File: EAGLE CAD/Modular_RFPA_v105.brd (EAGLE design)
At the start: 152.4 x 152.4 mm, 197 parts, among them IC201 74AHC1G14DBV, IC202 LM324D, J1 FUSE_2P, J2 KK_PCFAN, Q1 IRF630, Q101 IRF630, Q102 IRF520N, Q2 IRF630, Q201 BSS123, T1 HP4_TRAFO, T2 HP4_TRAFO, X101 HEATSINK_OMNI_DUAL30-75-D

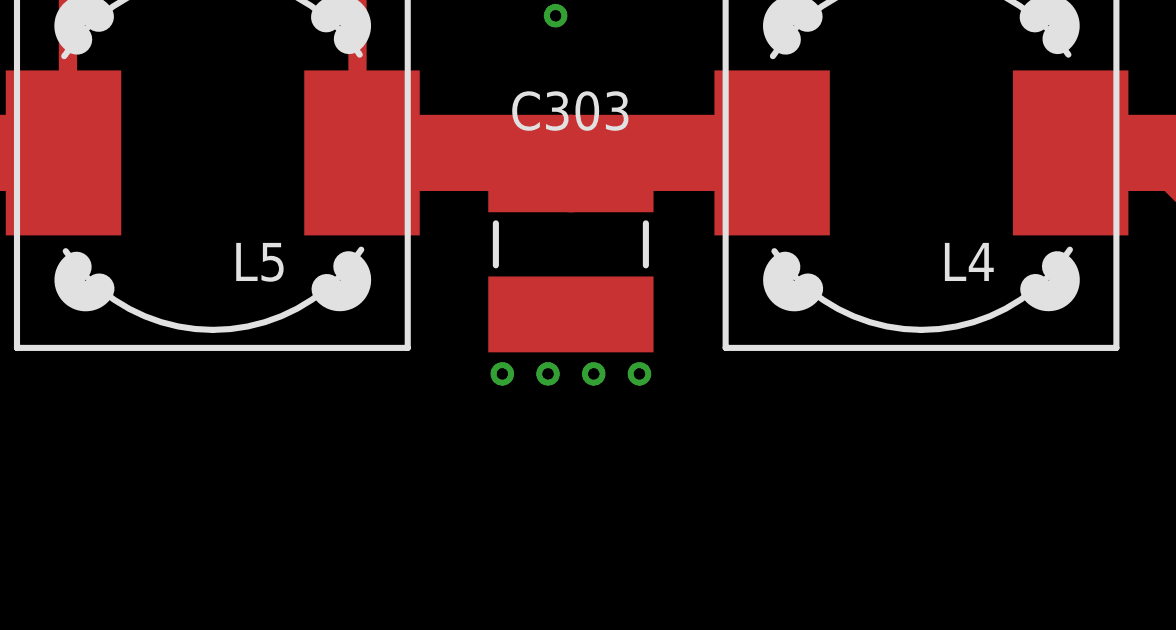
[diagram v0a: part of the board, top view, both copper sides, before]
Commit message: Work on libraries...
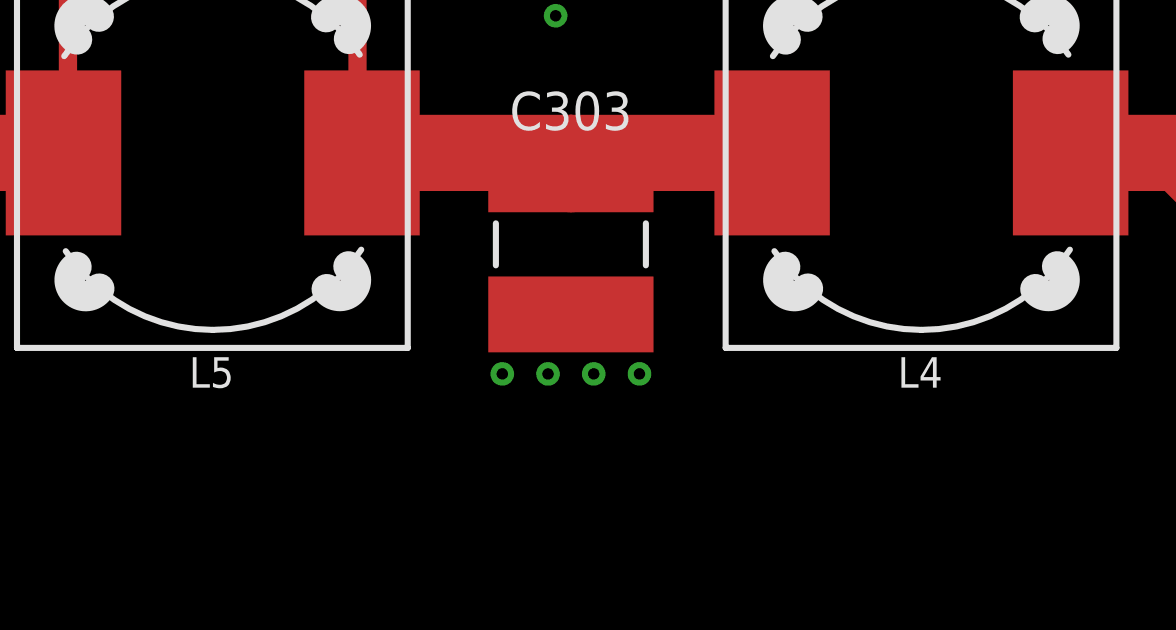
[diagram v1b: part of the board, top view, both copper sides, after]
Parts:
- C1, C111, C112, C7: value 2.2nF -> 22nF
- C102, C104, C12, C6: value 22nF -> 0.1uF
- C103, C11, C5: value 27nF -> 0.1uF
- C105: value 12nF -> 0.1uF
- C106, C107, C109, C110, C17, C207, C208, C24, C26, C27, C28: value DNP -> 0.1uF
- C113, C114, C2, C8: value 10nF -> 0.1uF
- C15, C16: value 4.7uF -> 47nF
- C209: value 15pF -> 0.1uF
- C25: value 1.5nF -> 0.1uF
- C29: value 100nF -> 0.1uF
- L1, L101, L2: value 47nH -> 1uH
- L102: value 150nH -> 1uH
- L4, L5: device inductors:DR127 -> MDT_L:DR127
- R1, R118, R120, R14: value 270 -> 1K
- R101, R105, R13, R18, R26, R5: value 75 -> 1K
- R102, R106: value 150 -> 1K
- R103, R19, R6: value 4.99 -> 1K
- R104: value 10 -> 1K
- R107, R109, R12, R218, R25: value 100 -> 1.0K
- R108, R110, R17, R4: value 100 -> 1K
- R111, R112, R115, R116, R211, R214: value DNP -> 1.0K
- R113, R114, R21, R8: value 15 -> 1.0K
- R117, R20, R7: value 330 -> 1K
- R119: value 2.74K -> 1K
- R121, R123, R15, R16, R2, R3, R34, R36, R38: value 2.7 -> 1K
- R122, R124: value 6.8 -> 1K
- R202, R203, R204, R205, R206, R212, R219: value 10K -> 1.0K
- R216, R30: value 0 -> 1.0K
- R217: value 10 -> 1.0K
- R302, R303, R40: value 1.0 -> 1K
- R32, R33: value 8.2 -> 1K
- R35, R37, R39: value 3.3 -> 1K
- R41: value 150 -> 1.0K
- R43: value 0.5 -> 1K
